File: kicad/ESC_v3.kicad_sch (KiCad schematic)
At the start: 29 parts, among them J1 Conn_01x05_Pin, J2 Conn_01x05_Pin, J4 Conn_01x06_Pin, J6 Conn_01x06_Pin, J7 Conn_01x02_Pin, J8 Conn_01x04_Pin, SW2 SW_Nidec_CAS-120A1, U10 BD4104, U14 MCP9700x-ETT, U16 AS5048A, U19 STM32G431CBUx

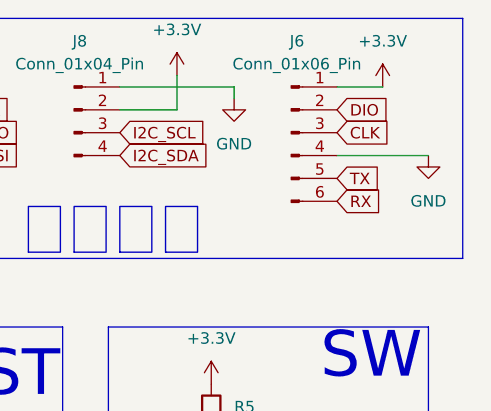
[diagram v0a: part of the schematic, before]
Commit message: final
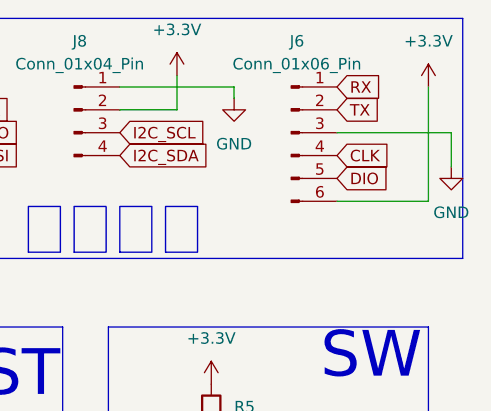
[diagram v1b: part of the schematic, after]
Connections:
- net +3.3V: now also J6.6 (Pin_6); no longer J6.1 (Pin_1)
- net CLK: now also J6.4 (Pin_4); no longer J6.3 (Pin_3)
- net DIO: now also J6.5 (Pin_5); no longer J6.2 (Pin_2)
- net GND: now also J6.3 (Pin_3); no longer J6.4 (Pin_4)
- net RX: now also J6.1 (Pin_1); no longer J6.6 (Pin_6)
- net TX: now also J6.2 (Pin_2); no longer J6.5 (Pin_5)
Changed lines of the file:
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@@
 	(wire
 		(pts
-			(xy 275.59 20.32) (xy 270.51 20.32)
-		)
-		(stroke
-			(width 0)
-			(type default)
-		)
-	)
-	(wire
-		(pts
 			(xy 172.72 144.78) (xy 172.72 149.86)
 		)
@@
 	(wire
 		(pts
+			(xy 283.21 29.21) (xy 283.21 25.4)
+		)
+		(stroke
+			(width 0)
+			(type default)
+		)
+	)
+	(wire
+		(pts
 			(xy 217.17 62.23) (xy 220.98 62.23)
 		)
@@
 	(wire
 		(pts
-			(xy 280.67 27.94) (xy 270.51 27.94)
+			(xy 280.67 33.02) (xy 270.51 33.02)
 		)
 		(stroke
@@
 	(wire
 		(pts
+			(xy 280.67 20.32) (xy 280.67 33.02)
+		)
+		(stroke
+			(width 0)
+			(type default)
+		)
+	)
+	(wire
+		(pts
 			(xy 262.89 71.12) (xy 262.89 72.39)
 		)
@@
 	(wire
 		(pts
+			(xy 283.21 25.4) (xy 270.51 25.4)
+		)
+		(stroke
+			(width 0)
+			(type default)
+		)
+	)
+	(wire
+		(pts
 			(xy 168.91 152.4) (xy 185.42 152.4)
 		)
@@
 		)
 	)
-	(global_label "RX"
-		(shape input)
-		(at 270.51 33.02 0)
-		(fields_autoplaced yes)
-		(effects
-			(font
-				(size 1.27 1.27)
-			)
-			(justify left)
-		)
-		(property "Intersheetrefs" "${INTERSHEET_REFS}"
-			(at 275.9747 33.02 0)
-			(effects
-				(font
-					(size 1.27 1.27)
-				)
-				(justify left)
-				(hide yes)
-			)
-		)
-	)
 	(global_label "TIM2_CH2"
 		(shape input)
@@
 		)
 	)
+	(global_label "TX"
+		(shape input)
+		(at 270.51 22.86 0)
+		(fields_autoplaced yes)
+		(effects
+			(font
+				(size 1.27 1.27)
+			)
+			(justify left)
+		)
+		(property "Intersheetrefs" "${INTERSHEET_REFS}"
+			(at 275.6723 22.86 0)
+			(effects
+				(font
+					(size 1.27 1.27)
+				)
+				(justify left)
+				(hide yes)
+			)
+		)
+	)
 	(global_label "CAN_L"
 		(shape input)
@@
 		)
 	)
-	(global_label "DIO"
-		(shape input)
-		(at 270.51 22.86 0)
-		(fields_autoplaced yes)
-		(effects
-			(font
-				(size 1.27 1.27)
-			)
-			(justify left)
-		)
-		(property "Intersheetrefs" "${INTERSHEET_REFS}"
-			(at 276.7005 22.86 0)
-			(effects
-				(font
-					(size 1.27 1.27)
-				)
-				(justify left)
-				(hide yes)
-			)
-		)
-	)
 	(global_label "TIM8_CH1"
 		(shape input)
@@
 		)
 	)
-	(global_label "CLK"
+	(global_label "ADC2_IN10"
 		(shape input)
-		(at 270.51 25.4 0)
+		(at 34.29 39.37 180)
 		(fields_autoplaced yes)
 		(effects
@@
 				(size 1.27 1.27)
 			)
-			(justify left)
+			(justify right)
 		)
 		(property "Intersheetrefs" "${INTERSHEET_REFS}"
-			(at 277.0633 25.4 0)
+			(at 21.1448 39.37 0)
 			(effects
 				(font
 					(size 1.27 1.27)
 				)
-				(justify left)
+				(justify right)
 				(hide yes)
 			)
 		)
 	)
-	(global_label "ADC2_IN10"
+	(global_label "DIO"
 		(shape input)
-		(at 34.29 39.37 180)
+		(at 270.51 30.48 0)
 		(fields_autoplaced yes)
 		(effects
@@
 				(size 1.27 1.27)
 			)
-			(justify right)
+			(justify left)
 		)
 		(property "Intersheetrefs" "${INTERSHEET_REFS}"
-			(at 21.1448 39.37 0)
+			(at 276.7005 30.48 0)
 			(effects
 				(font
 					(size 1.27 1.27)
 				)
-				(justify right)
+				(justify left)
 				(hide yes)
 			)
@@
 		)
 	)
-	(global_label "TX"
-		(shape input)
-		(at 270.51 30.48 0)
-		(fields_autoplaced yes)
-		(effects
-			(font
-				(size 1.27 1.27)
-			)
-			(justify left)
-		)
-		(property "Intersheetrefs" "${INTERSHEET_REFS}"
-			(at 275.6723 30.48 0)
-			(effects
-				(font
-					(size 1.27 1.27)
-				)
-				(justify left)
-				(hide yes)
-			)
-		)
-	)
 	(global_label "CAN_L"
 		(shape input)
@@
 		)
 	)
+	(global_label "CLK"
+		(shape input)
+		(at 270.51 27.94 0)
+		(fields_autoplaced yes)
+		(effects
+			(font
+				(size 1.27 1.27)
+			)
+			(justify left)
+		)
+		(property "Intersheetrefs" "${INTERSHEET_REFS}"
+			(at 277.0633 27.94 0)
+			(effects
+				(font
+					(size 1.27 1.27)
+				)
+				(justify left)
+				(hide yes)
+			)
+		)
+	)
 	(global_label "TIM2_CH1"
 		(shape input)
@@
 		)
 	)
+	(global_label "RX"
+		(shape input)
+		(at 270.51 20.32 0)
+		(fields_autoplaced yes)
+		(effects
+			(font
+				(size 1.27 1.27)
+			)
+			(justify left)
+		)
+		(property "Intersheetrefs" "${INTERSHEET_REFS}"
+			(at 275.9747 20.32 0)
+			(effects
+				(font
+					(size 1.27 1.27)
+				)
+				(justify left)
+				(hide yes)
+			)
+		)
+	)
 	(global_label "SPI1_MISO"
 		(shape input)
@@
 	(symbol
 		(lib_id "power:GND")
-		(at 280.67 27.94 0)
+		(at 283.21 29.21 0)
 		(unit 1)
 		(exclude_from_sim no)
@@
 		(fields_autoplaced yes)
 		(property "Reference" "#PWR028"
-			(at 280.67 34.29 0)
+			(at 283.21 35.56 0)
 			(effects
 				(font
@@
 		)
 		(property "Value" "GND"
-			(at 280.67 33.02 0)
+			(at 283.21 34.29 0)
 			(effects
 				(font
@@
 		)
 		(property "Footprint" ""
-			(at 280.67 27.94 0)
+			(at 283.21 29.21 0)
 			(effects
 				(font
@@
 		)
 		(property "Datasheet" ""
-			(at 280.67 27.94 0)
+			(at 283.21 29.21 0)
 			(effects
 				(font
@@
 		)
 		(property "Description" "Power symbol creates a global label with name \"GND\" , ground"
-			(at 280.67 27.94 0)
+			(at 283.21 29.21 0)
 			(effects
 				(font
@@
 	(symbol
 		(lib_id "power:+3.3V")
-		(at 275.59 20.32 0)
+		(at 280.67 20.32 0)
 		(unit 1)
 		(exclude_from_sim no)
@@
 		(fields_autoplaced yes)
 		(property "Reference" "#PWR049"
-			(at 275.59 24.13 0)
+			(at 280.67 24.13 0)
 			(effects
 				(font
@@
 		)
 		(property "Value" "+3.3V"
-			(at 275.59 15.24 0)
+			(at 280.67 15.24 0)
 			(effects
 				(font
@@
 		)
 		(property "Footprint" ""
-			(at 275.59 20.32 0)
+			(at 280.67 20.32 0)
 			(effects
 				(font
@@
 		)
 		(property "Datasheet" ""
-			(at 275.59 20.32 0)
+			(at 280.67 20.32 0)
 			(effects
 				(font
@@
 		)
 		(property "Description" "Power symbol creates a global label with name \"+3.3V\""
-			(at 275.59 20.32 0)
+			(at 280.67 20.32 0)
 			(effects
 				(font
